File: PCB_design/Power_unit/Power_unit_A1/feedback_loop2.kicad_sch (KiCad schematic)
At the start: 5 parts, among them U1502 DAC70501MDQFR

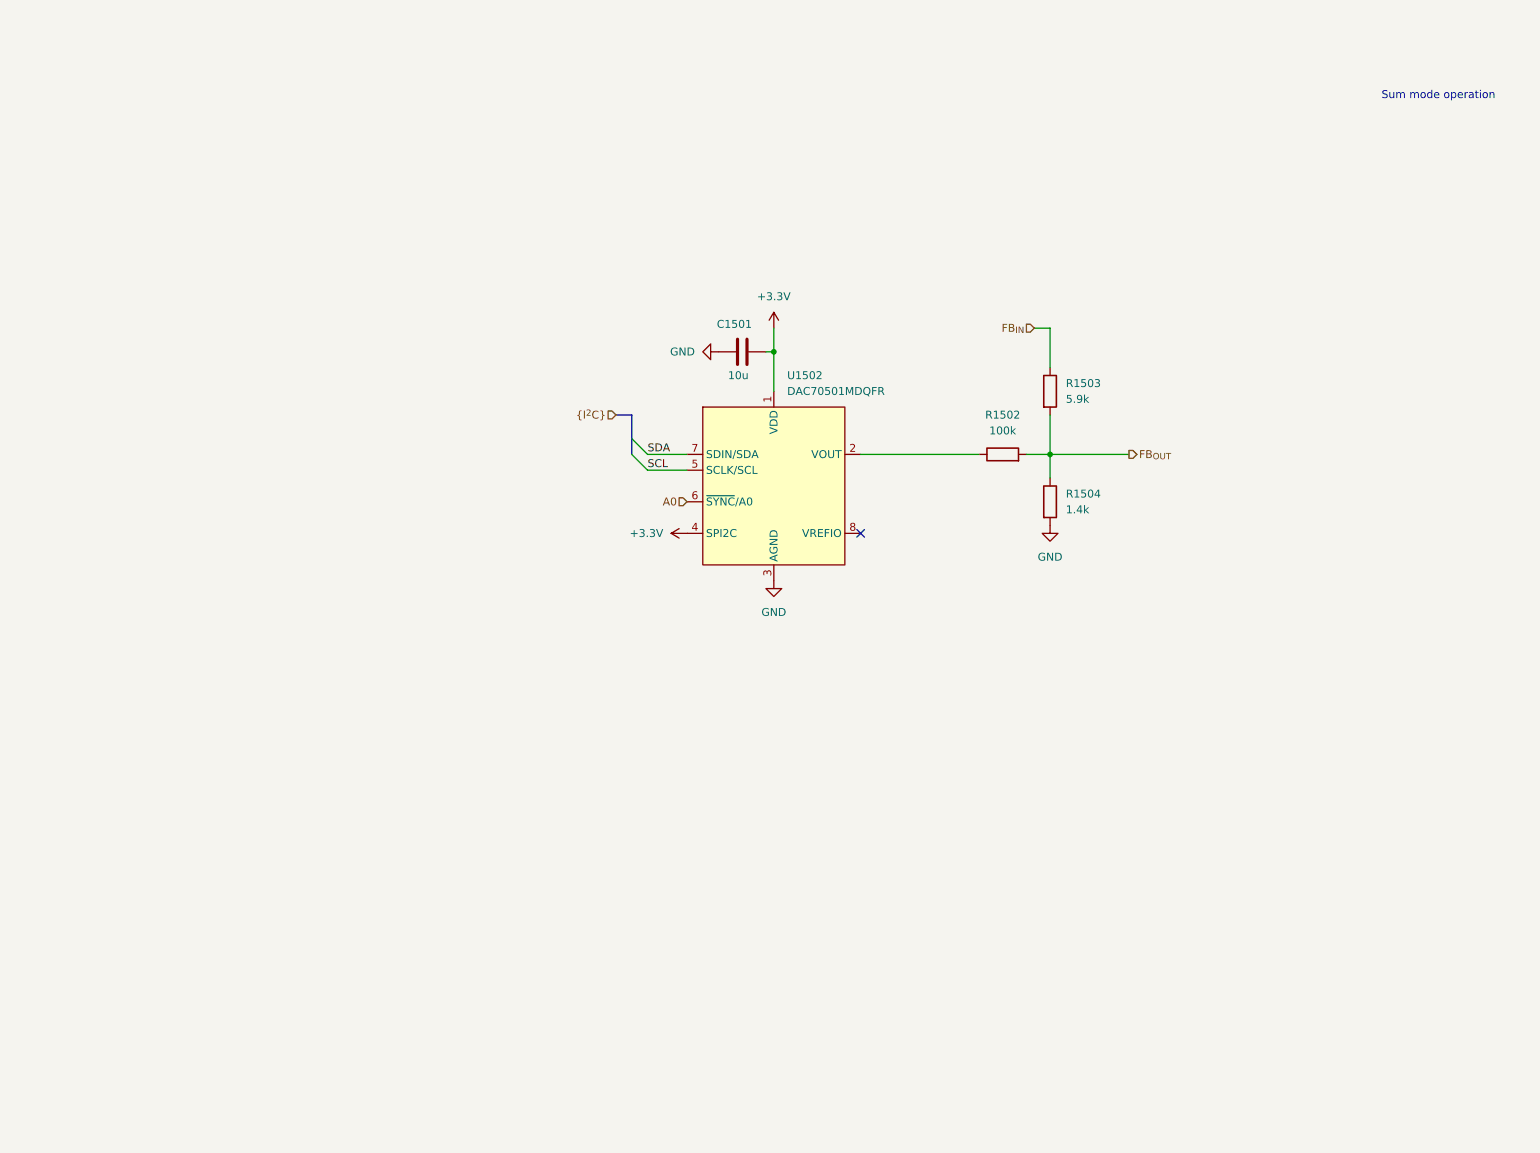
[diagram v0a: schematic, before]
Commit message: WIP
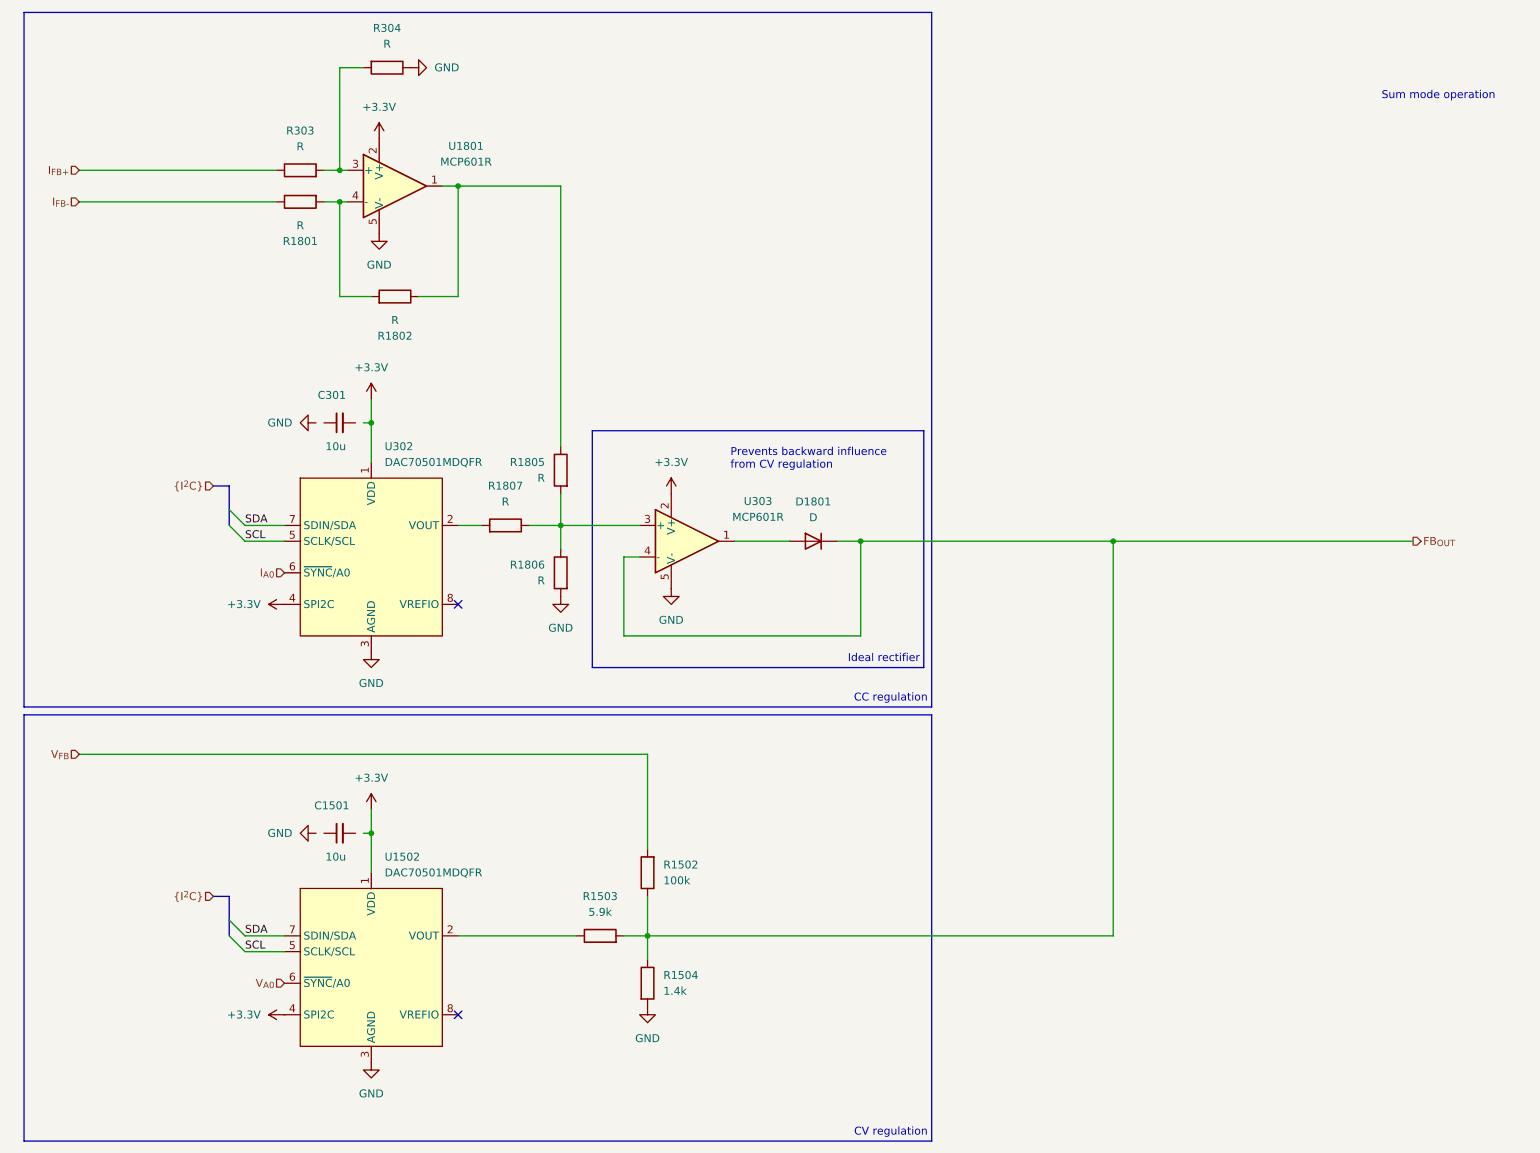
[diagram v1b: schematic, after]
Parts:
- added C301: 10u, symbol Device:C_Small
- added D1801: D, symbol Device:D
- added R1801, R1802, R1805, R1806, R1807, R303, R304: R, symbol Device:R
- added U1801, U303: MCP601R, Package_TO_SOT_SMD:SOT-23-5, symbol Amplifier_Operational:MCP601R
- added U302: DAC70501MDQFR, Power_supply:Texas_DQF0008A_WSON-8_2x2mm_P0.8mm, symbol Power_supply:DAC70501MDQFR
- C1501: symbol Device:C -> Device:C_Small
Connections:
- net FB_{IN} is gone; now on an unnamed net: R1503.1
- net +3.3V: now also U1801.2 (V+), U302.1 (VDD), U302.4 (SPI2C), U303.2 (V+); no longer C1501.2
- net FB_{OUT}: now also R1502.1, D1801.1 (K), U303.4 (-); no longer R1502.2
- net GND: now also R1806.2, R304.1, U1801.5 (V-), U302.3 (AGND), U303.5 (V-); no longer C1501.1
- net SCL: now also U302.5 (SCLK/SCL)
- net SDA: now also U302.7 (SDIN/SDA)
- net at U1502.2 (VOUT): no longer R1502.1
- net A0 renamed V_{A0}
- new net: R303.2, R304.2, U1801.3 (+)
- new net: D1801.2 (A), U303.1
- new net: R1805.2, R1806.1, R1807.1, U303.3 (+)
- new net: R1802.1, R1805.1, U1801.1
- new net: R1807.2, U302.2 (VOUT)
- new net: R1801.2, R1802.2, U1801.4 (-)
- new net I_{A0}: U302.6 (~{SYNC}/A0)
- new net I_{FB+}: R303.1
- new net I_{FB-}: R1801.1
- new net V_{FB}: R1502.2
- no-connect marks 1 -> 2
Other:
- note added: "CC regulation"
- note added: "CV regulation"
- note added: "Ideal rectifier"
- note added: "Prevents backward influence from CV regulation"
- company: (none) -> David Haisman
- title: (none) -> ${PROJECTNAME}
- moved on the sheet: C1501, R1502, R1503, R1504, U1502
